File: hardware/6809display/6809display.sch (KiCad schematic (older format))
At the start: 43 parts, among them J1 Video Out, J2 To Computer, Q1 BC557, Q2 BC557, Q3 BC557, U1 74HC04, U10 74HC283, U2 74HC04, U3 74HC393, U4 SAA5020, U5 SAA5050, U6 IDT7132, U7 74HC08, U8 74HC283, U9 74HC283, Y1 6MHz

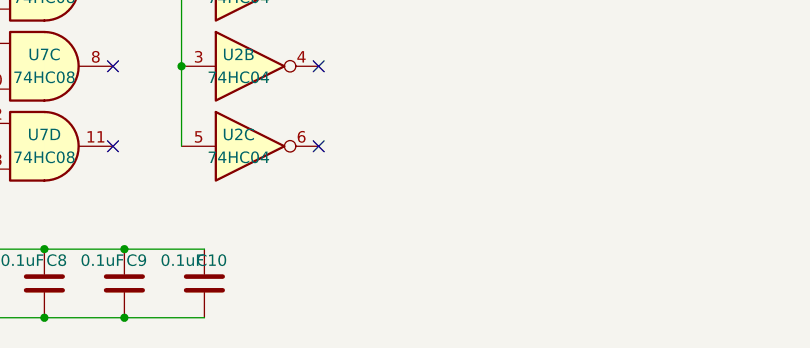
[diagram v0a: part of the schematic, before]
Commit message: expansion board
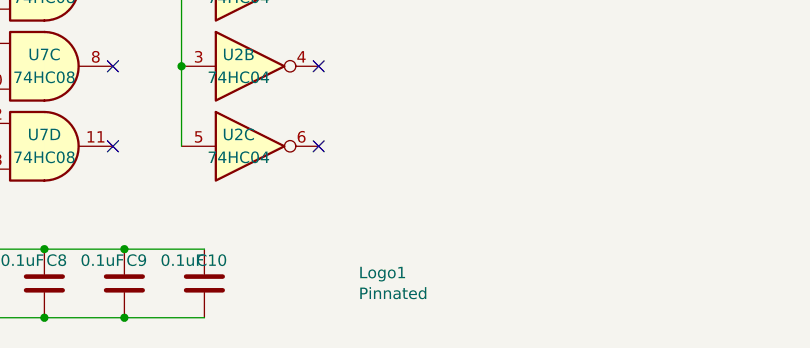
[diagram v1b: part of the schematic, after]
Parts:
- added Logo1: Pinnated, Pinnated:Pinnule, symbol aspt:Pinnated
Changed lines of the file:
@@
 Wire Bus Line
 	15650 1150 15650 3150
+$Comp
+L aspt:Pinnated Logo1
+U 1 1 60AA09D0
+P 4950 10700
+F 0 "Logo1" H 4975 10746 50  0000 L CNN
+F 1 "Pinnated" H 4975 10655 50  0000 L CNN
+F 2 "Pinnated:Pinnule" H 4950 10700 50  0001 C CNN
+F 3 "" H 4950 10700 50  0001 C CNN
+	1    4950 10700
+	1    0    0    -1
+$EndComp
 $EndSCHEMATC
